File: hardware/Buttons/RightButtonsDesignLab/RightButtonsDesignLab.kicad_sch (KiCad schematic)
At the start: 5 parts, among them J1 Conn_01x03, J2 Conn_01x01, SW1 SW_Push, SW2 SW_Push, SW3 SW_Push

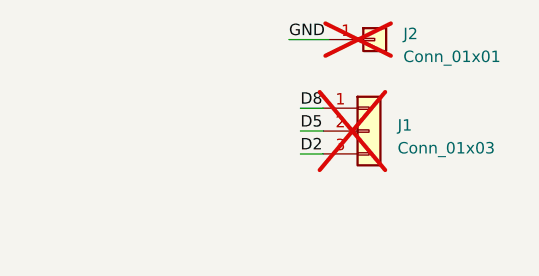
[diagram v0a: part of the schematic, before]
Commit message: Update all PCB and schematics
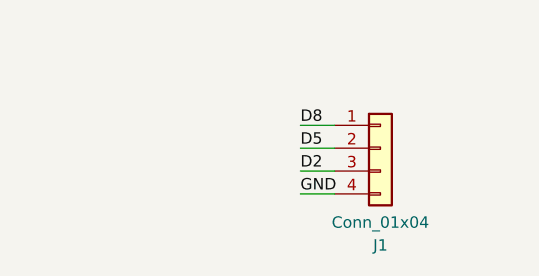
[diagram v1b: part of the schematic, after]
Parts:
- removed J1: Conn_01x03, Connector_PinHeader_2.54mm:PinHeader_1x03_P2.54mm_Vertical, symbol Connector_Generic:Conn_01x03
- removed J2: Conn_01x01, Connector_PinHeader_2.54mm:PinHeader_1x01_P2.54mm_Vertical, symbol Connector_Generic:Conn_01x01
- added J1: Conn_01x04, Design:JST_S4B-PH-K-S_LF__SN_, symbol Connector_Generic:Conn_01x04
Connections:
- net D2: now also J1.3 (Pin_3)
- net D5: now also J1.2 (Pin_2)
- net D8: now also J1.1 (Pin_1)
- net GND: now also J1.4 (Pin_4)
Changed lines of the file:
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@@
 (kicad_sch (version 20230121) (generator eeschema)
   (paper "A4")
-  (wire (pts (xy 180.34 23.495) (xy 184.785 23.495))
+  (wire (pts (xy 27.94 37.465) (xy 34.29 37.465))
     (stroke (width 0) (type default))
   )
-  (wire (pts (xy 27.94 37.465) (xy 34.29 37.465))
+  (wire (pts (xy 181.61 38.1) (xy 185.42 38.1))
+    (stroke (width 0) (type default))
+  )
+  (wire (pts (xy 181.61 33.02) (xy 185.42 33.02))
     (stroke (width 0) (type default))
   )
@@
     (stroke (width 0) (type default))
   )
-  (wire (pts (xy 181.61 33.655) (xy 184.15 33.655))
+  (wire (pts (xy 69.215 37.465) (xy 75.565 37.465))
     (stroke (width 0) (type default))
   )
-  (wire (pts (xy 69.215 37.465) (xy 75.565 37.465))
+  (wire (pts (xy 181.61 35.56) (xy 185.42 35.56))
     (stroke (width 0) (type default))
   )
@@
     (stroke (width 0) (type default))
   )
-  (wire (pts (xy 181.61 31.115) (xy 184.15 31.115))
-    (stroke (width 0) (type default))
-  )
-  (wire (pts (xy 181.61 36.195) (xy 184.15 36.195))
+  (wire (pts (xy 181.61 40.64) (xy 185.42 40.64))
     (stroke (width 0) (type default))
   )
@@
     (effects (font (size 1.27 1.27)) (justify left bottom))
   )
-  (label "GND" (at 27.94 37.465 0) (fields_autoplaced)
+  (label "D2" (at 181.61 38.1 0) (fields_autoplaced)
     (effects (font (size 1.27 1.27)) (justify left bottom))
   )
-  (label "GND" (at 180.34 23.495 0) (fields_autoplaced)
+  (label "D5" (at 181.61 35.56 0) (fields_autoplaced)
     (effects (font (size 1.27 1.27)) (justify left bottom))
   )
-  (label "D2" (at 181.61 36.195 0) (fields_autoplaced)
+  (label "GND" (at 27.94 37.465 0) (fields_autoplaced)
     (effects (font (size 1.27 1.27)) (justify left bottom))
   )
@@
     (effects (font (size 1.27 1.27)) (justify left bottom))
   )
-  (label "D5" (at 181.61 33.655 0) (fields_autoplaced)
-    (effects (font (size 1.27 1.27)) (justify left bottom))
-  )
   (label "D2" (at 46.99 37.465 0) (fields_autoplaced)
     (effects (font (size 1.27 1.27)) (justify left bottom))
   )
-  (label "D8" (at 181.61 31.115 0) (fields_autoplaced)
+  (label "D8" (at 125.095 37.465 0) (fields_autoplaced)
     (effects (font (size 1.27 1.27)) (justify left bottom))
   )
-  (label "D8" (at 125.095 37.465 0) (fields_autoplaced)
+  (label "D8" (at 181.61 33.02 0) (fields_autoplaced)
+    (effects (font (size 1.27 1.27)) (justify left bottom))
+  )
+  (label "GND" (at 181.61 40.64 0) (fields_autoplaced)
     (effects (font (size 1.27 1.27)) (justify left bottom))
   )
@@
     )
   )
-  (symbol (lib_id "Connector_Generic:Conn_01x03") (at 189.23 33.655 0) (unit 1)
-    (in_bom yes) (on_board yes) (dnp yes) (fields_autoplaced)
-    (property "Reference" "J1" (at 192.405 33.02 0)
-      (effects (font (size 1.27 1.27)) (justify left))
+  (symbol (lib_id "Connector_Generic:Conn_01x04") (at 190.5 35.56 0) (unit 1)
+    (in_bom yes) (on_board yes) (dnp no)
+    (property "Reference" "J1" (at 190.5 46.355 0)
+      (effects (font (size 1.27 1.27)))
     )
-    (property "Value" "Conn_01x03" (at 192.405 35.56 0)
-      (effects (font (size 1.27 1.27)) (justify left))
+    (property "Value" "Conn_01x04" (at 190.5 43.815 0)
+      (effects (font (size 1.27 1.27)))
     )
-    (property "Footprint" "Connector_PinHeader_2.54mm:PinHeader_1x03_P2.54mm_Vertical" (at 189.23 33.655 0)
+    (property "Footprint" "Design:JST_S4B-PH-K-S_LF__SN_" (at 190.5 35.56 0)
       (effects (font (size 1.27 1.27)) hide)
     )
-    (property "Datasheet" "~" (at 189.23 33.655 0)
+    (property "Datasheet" "https://datasheet.lcsc.com/lcsc/2304140030_JST-S4B-PH-K-S-LF-SN_C157926.pdf" (at 190.5 35.56 0)
+      (effects (font (size 1.27 1.27)) hide)
+    )
+    (property "LCSC#" "C157926" (at 190.5 35.56 0)
       (effects (font (size 1.27 1.27)) hide)
     )
@@
     (pin "2")
     (pin "3")
+    (pin "4")
     (instances
       (project "RightButtonsDesignLab"
@@
         )
       )
-      (project "ButtonDesignLab"
-        (path "/e63e39d7-6ac0-4ffd-8aa3-1841a4541b55"
-          (reference "J2") (unit 1)
-        )
-      )
-    )
-  )
-  (symbol (lib_id "Connector_Generic:Conn_01x01") (at 189.865 23.495 0) (unit 1)
-    (in_bom yes) (on_board yes) (dnp yes) (fields_autoplaced)
-    (property "Reference" "J2" (at 193.04 22.86 0)
-      (effects (font (size 1.27 1.27)) (justify left))
-    )
-    (property "Value" "Conn_01x01" (at 193.04 25.4 0)
-      (effects (font (size 1.27 1.27)) (justify left))
-    )
-    (property "Footprint" "Connector_PinHeader_2.54mm:PinHeader_1x01_P2.54mm_Vertical" (at 189.865 23.495 0)
-      (effects (font (size 1.27 1.27)) hide)
-    )
-    (property "Datasheet" "~" (at 189.865 23.495 0)
-      (effects (font (size 1.27 1.27)) hide)
-    )
-    (pin "1")
-    (instances
-      (project "RightButtonsDesignLab"
-        (path "/d8ab91b7-7f4a-4c3a-afb3-beb7d8cda53a"
-          (reference "J2") (unit 1)
-        )
-      )
-      (project "ButtonDesignLab"
-        (path "/e63e39d7-6ac0-4ffd-8aa3-1841a4541b55"
-          (reference "J7") (unit 1)
-        )
-      )
